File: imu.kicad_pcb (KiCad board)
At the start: 2 copper layers, 50 parts, among them IC1 ATTINY2313-S, IC2 ATTINY2313-S, K1 AIN0, P1 GPS-ANT, P2 MB77.07, P3 CONN_5, P4 CONN_4, P5 CONN_5, P6 CONN_10, P7 CONN_5, P8 CONN_10, P9 GPIO, SW1 RESET, U1 PCF8574, X1 CRYSTAL, X2 CRYSTAL

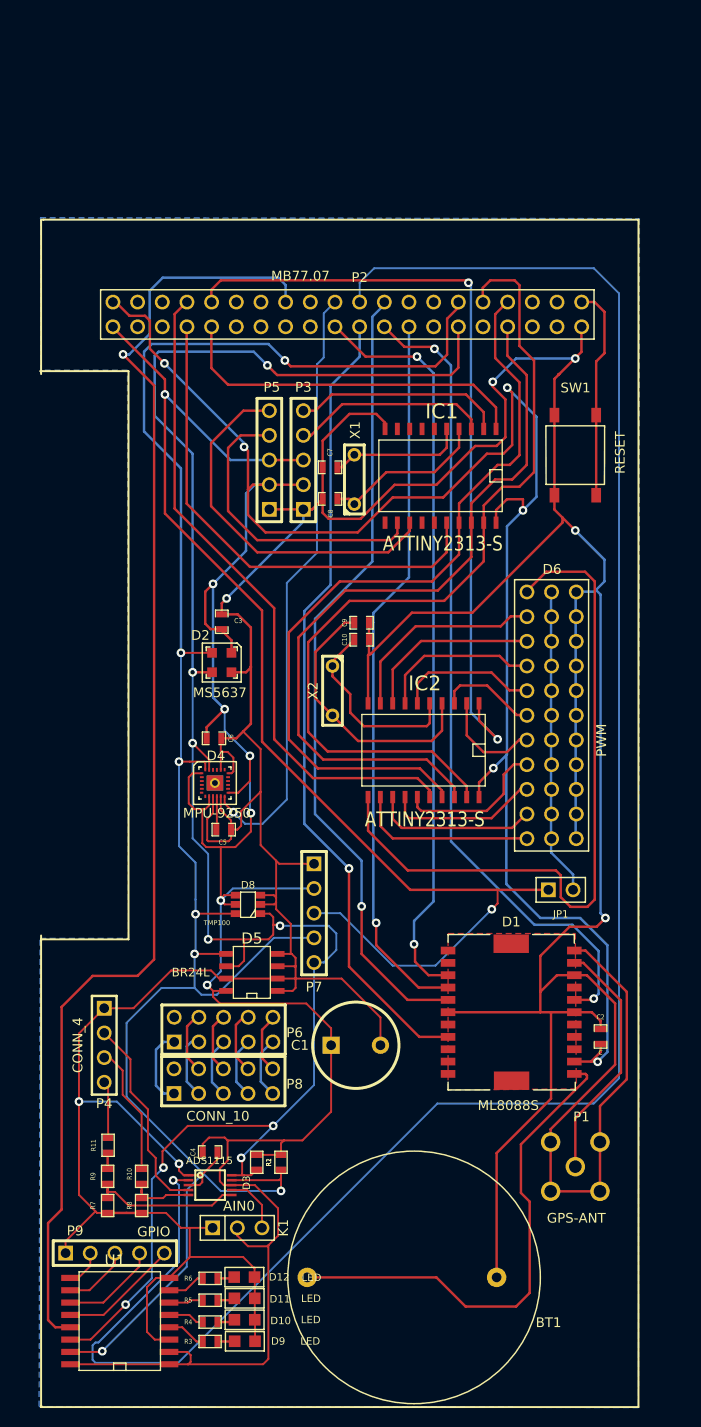
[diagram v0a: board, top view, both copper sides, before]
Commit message: pcb and elements
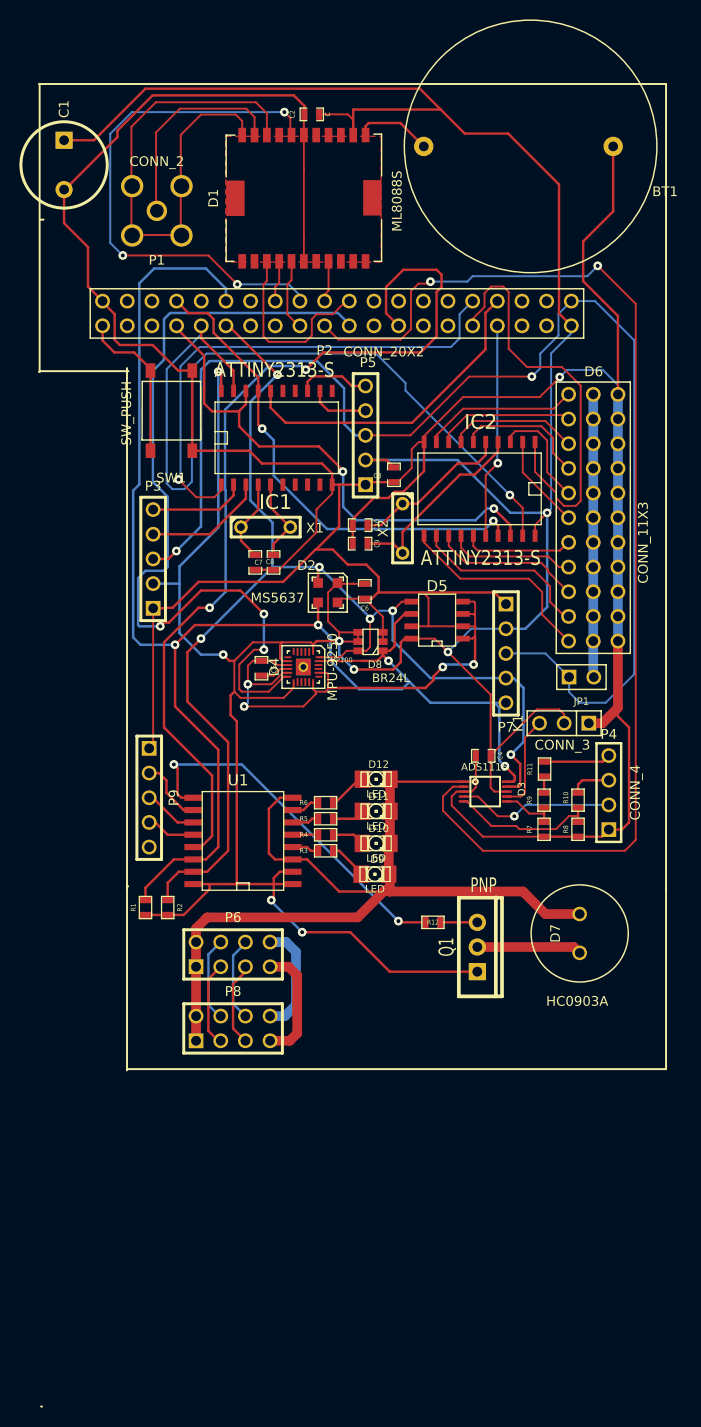
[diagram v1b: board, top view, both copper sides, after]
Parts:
- added D7: HC0903A, HC0903A, F.Cu at (68.5, 102.5)
- added Q1: PNP, TO220_VERT, F.Cu at (57.9, 103.9)
- added R12: R, SM0603, F.Cu at (53.3, 101.3)
- D10, D11, D12, D9: footprint led0805 -> LED-1206
- D6: value PWM -> CONN_11X3
- K1: value AIN0 -> CONN_3
- P1: value GPS-ANT -> CONN_2
- P2: value MB77.07 -> CONN_20X2
- P6, P8: value CONN_10 -> CONN_4X2; footprint PIN_ARRAY_5x2 -> pin_array_4x2
- P9: value GPIO -> CONN_4
- SW1: value RESET -> SW_PUSH
- moved BT1 117.1 mm to (63.4, 21.5)
- moved P1 107.4 mm to (24.9, 28.1), turned to 0 degrees
- moved C2 99.5 mm to (40.9, 18.2), turned to 180 degrees
- moved C1 95.5 mm to (15.4, 23.4), turned to 270 degrees
- moved D1 86.5 mm to (40.1, 26.8), turned to 90 degrees
- moved K1 61.9 mm to (66.9, 80.8), turned to 180 degrees
- moved R10 59.3 mm to (68.3, 88.8)
- moved R11 59.3 mm to (64.8, 85.6)
- moved R7 59.3 mm to (64.8, 91.8)
- moved R8 59.3 mm to (68.3, 91.8)
- moved R9 59.3 mm to (64.8, 88.8)
- moved P4 58.1 mm to (71.5, 88.0), turned to 90 degrees
- moved D12 53.0 mm to (47.5, 86.6)
- moved D11 51.9 mm to (47.5, 89.9)
- moved R3 51.9 mm to (42.3, 94.0)
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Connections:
- D1 pad 20: /GND -> N-0000021
- D1 pad 22: /GND -> N-0000021
- D6 pad 1: N-0000015 -> N-0000023
- D6 pad 10: N-0000017 (its old number) -> N-0000014
- D6 pad 19: N-0000011 -> N-0000024
- D6 pad 22: N-0000019 (its old number) -> N-0000011
- D6 pad 25: N-0000010 -> N-0000048
- D6 pad 28: N-0000022 -> N-0000010
- D6 pad 31: N-000009 (its old number) -> N-0000016
- D6 pad 4: N-0000018 (its old number) -> N-0000015
- D6 pad 7: N-0000014 -> N-0000022
- IC1 pad 17: /MISO -> /MOSI
- IC1 pad 18: /MOSI -> /MISO
- IC2 pad 11: N-0000015 -> N-0000016
- IC2 pad 12: N-000009 (its old number) -> N-0000010
- IC2 pad 13: N-0000022 -> N-0000048
- IC2 pad 14: N-0000010 -> N-0000011
- IC2 pad 15: N-0000019 (its old number) -> N-0000024
- IC2 pad 17: /MISO -> /MOSI
- IC2 pad 18: /MOSI -> /MISO
- IC2 pad 2: N-0000011 -> N-0000012
- IC2 pad 3: N-0000012 -> N-0000013
- IC2 pad 6: N-0000013 -> N-0000014
- IC2 pad 7: N-0000017 (its old number) -> N-0000022
- IC2 pad 8: N-0000014 -> N-0000015
- IC2 pad 9: N-0000018 (its old number) -> N-0000023
- P1 pad 1: /GND -> N-0000021
- P6 pad 1: N-0000027 (its old number) -> /GND
- P6 pad 2: (no net) -> /GND
- P8 pad 1: N-0000027 (its old number) -> /GND
- P8 pad 2: (no net) -> /GND
- P9 pad 3: N-0000047 (its old number) -> N-0000030
- P9 pad 4: N-0000050 (its old number) -> N-0000031
- P9 pad 5: N-0000048 -> (no net)
- U1 pad 10: N-0000047 (its old number) -> N-0000046
- U1 pad 11: N-0000050 (its old number) -> N-0000030
- U1 pad 12: N-0000048 -> N-0000031
- U1 pad 9: N-0000046 -> N-0000045
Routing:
- net /ADC_RDY: track 201.9 -> 120.9 mm, vias 1 -> 2
- net /GPS_STATUS: track 83.3 -> 4.26 mm, vias 1 -> 0
- net N-000009: track 82.9 -> 7.42 mm, vias 1 -> 0
- net /SDA: track 205.1 -> 131.8 mm, vias 7 -> 6
- net N-000004: track 74.5 -> 4.26 mm, vias 1 -> 0
- net N-0000015: track 72.7 -> 14.1 mm
- net /GPS_PPS: track 77.6 -> 19.7 mm, vias 2 -> 0
- net N-0000021: track 0.00 -> 53.2 mm
- net /CS1: track 68.7 -> 22.2 mm, vias 0 -> 1
- net N-000006: track 51.7 -> 8.05 mm
- net /GND: track 541.7 -> 501.0 mm, vias 7 -> 5
- net /GPIO_INT: track 135.3 -> 94.6 mm, vias 1 -> 2
- net /SCL: track 196.0 -> 155.6 mm, vias 9 -> 4
- net /RST1: track 81.0 -> 43.3 mm, vias 2 -> 0
- net N-0000045: track 0.00 -> 37.7 mm, vias 0 -> 2
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- removed copper zone on B.Cu, net /GND
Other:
- net class Default: via_drill 0.6 -> 0.4
- rule via_min_drill: 0.508 -> 0.4
